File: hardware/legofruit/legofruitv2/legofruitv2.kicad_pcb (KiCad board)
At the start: 2 copper layers, 7.5 x 2 mm, 47 parts, among them J1 Conn_01x06, J10 SERVO4, J11 Conn_01x03, J12 MOTOR1, J2 USB_B_Micro, J3 Conn_ARM_JTAG_SWD_10, J4 MOTOR2, J5 SERVO1, J6 SERVO2, J7 SERVO3, J8 UART, J9 POWER, Q1 DMG2305, U1 MDBT50Q-1MV2, U2 MOTOR2_DRV, U4 AP2112K-3.3, U5 MOTOR1_DRV, Y1 32768 KHz

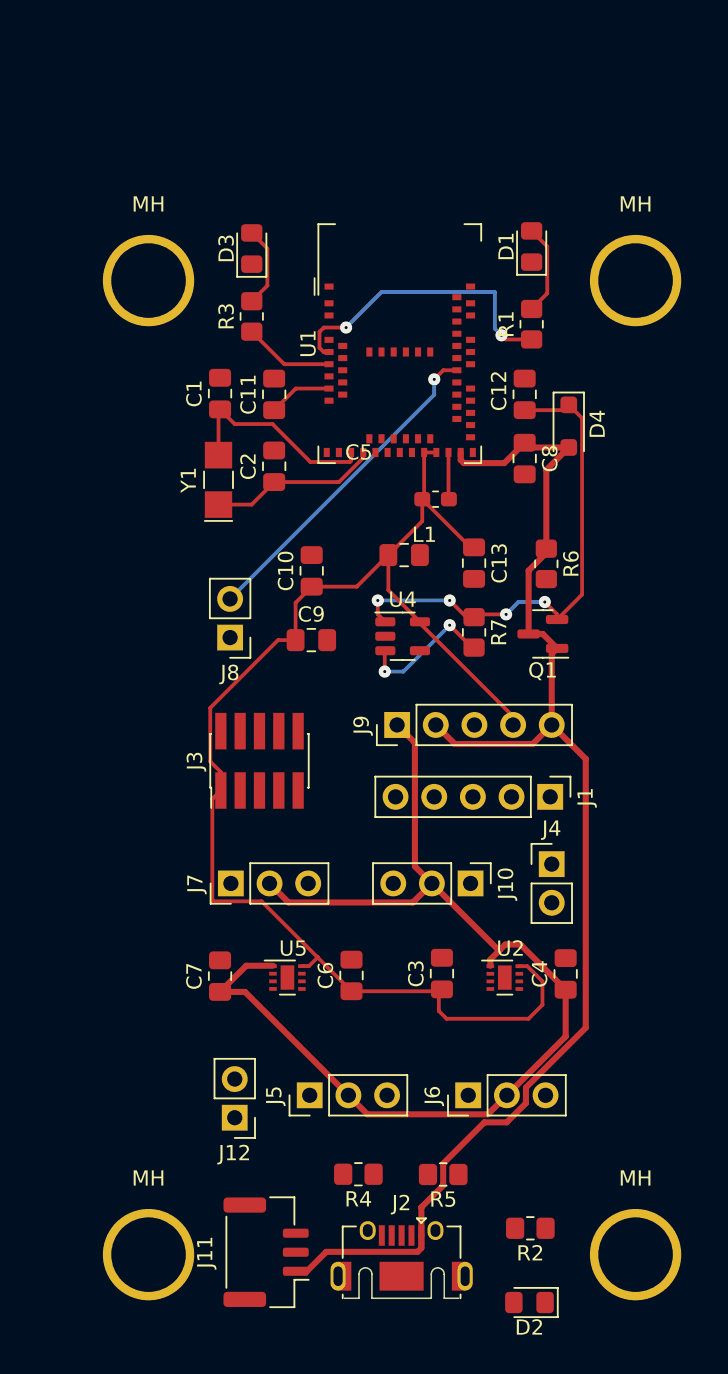
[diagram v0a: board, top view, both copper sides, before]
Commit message: Device driver version
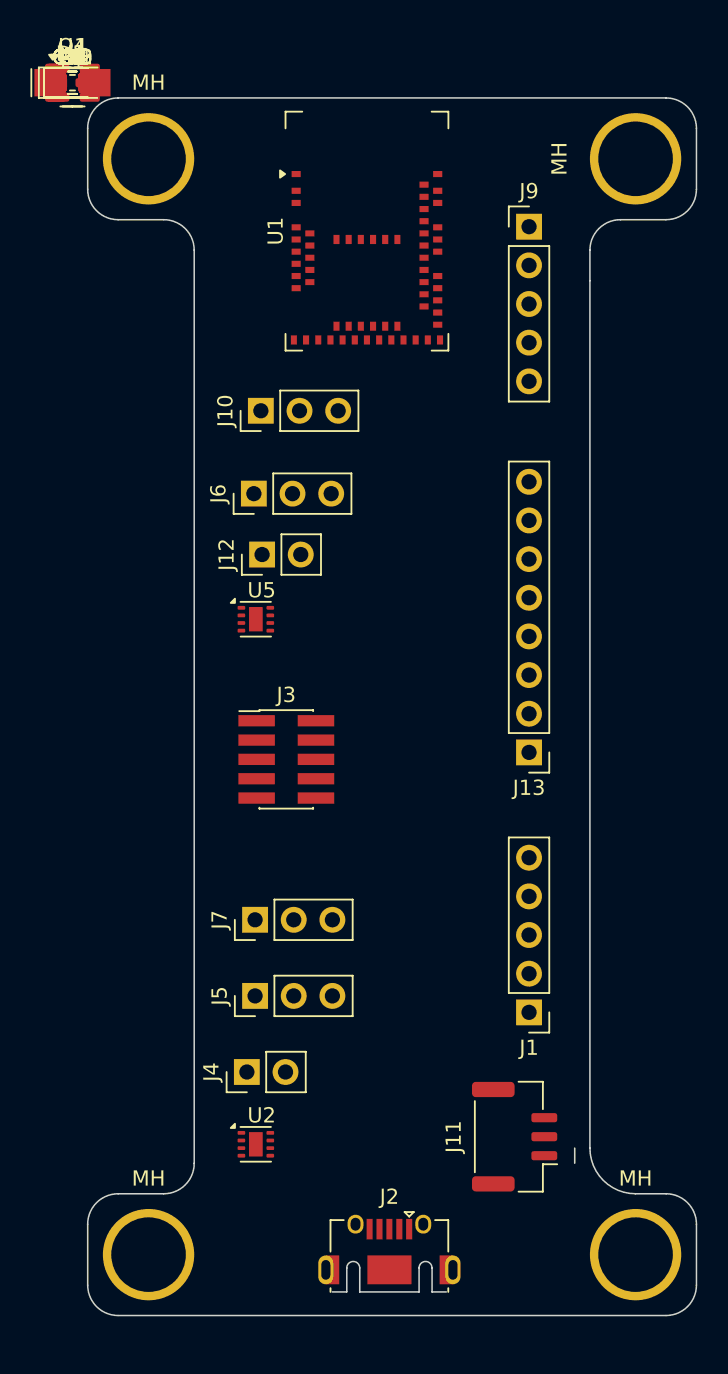
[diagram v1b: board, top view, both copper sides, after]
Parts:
- removed J8: UART, Connector_PinHeader_2.54mm:PinHeader_1x02_P2.54mm_Vertical
- added J13: GPIO, Connector_PinHeader_2.54mm:PinHeader_1x08_P2.54mm_Vertical, F.Cu at (125.0, 81.0)
- moved D2 85.6 mm to (95.0, 37.0), turned to 0 degrees
- moved R2 81.1 mm to (95.0, 37.0), turned to 0 degrees
- moved R5 75.8 mm to (95.0, 37.0), turned to 0 degrees
- moved R4 74.1 mm to (95.0, 37.0), turned to 0 degrees
- moved C4 66.9 mm to (95.0, 37.0), turned to 0 degrees
- moved C3 63.4 mm to (95.0, 37.0), turned to 0 degrees
- moved C6 61.5 mm to (95.0, 37.0), turned to 0 degrees
- moved C7 59.5 mm to (95.0, 37.0), turned to 0 degrees
- moved Q1 47.6 mm to (95.0, 37.0), turned to 0 degrees
- moved R7 44.7 mm to (95.0, 37.0), turned to 0 degrees
- moved R6 44.4 mm to (95.0, 37.0), turned to 0 degrees
- moved U4 42.3 mm to (95.0, 37.0)
- moved J6 42.0 mm to (106.9, 64.0)
- moved C13 41.1 mm to (95.0, 37.0), turned to 0 degrees
- moved C9 39.8 mm to (95.0, 37.0)
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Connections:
- U1 pad 43: Net-(J8-Pin_2) -> unconnected-(U1-P0.21-Pad43)
- U1 pad 44: Net-(J8-Pin_1) -> unconnected-(U1-P0.20-Pad44)
- U1 pad 50: unconnected-(U1-P1.02-Pad50) -> Net-(J13-Pin_5)
- U1 pad 56: unconnected-(U1-P1.04-Pad56) -> Net-(J13-Pin_3)
- U1 pad 57: unconnected-(U1-P1.06-Pad57) -> Net-(J13-Pin_1)
- U1 pad 59: unconnected-(U1-P1.05-Pad59) -> Net-(J13-Pin_2)
- U1 pad 60: unconnected-(U1-P1.03-Pad60) -> Net-(J13-Pin_4)
- U1 pad 61: unconnected-(U1-P1.01-Pad61) -> Net-(J13-Pin_6)
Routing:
- net +3.3V: track 89.5 -> 0.00 mm
- net VBUS: track 87.3 -> 0.00 mm
- net VCC: track 71.8 -> 0.00 mm
- net Net-(D4-K): track 33.1 -> 0.00 mm, vias 4 -> 0
- net Net-(J8-Pin_2): track 21.7 -> 0.00 mm, vias 1 -> 0
- net /P1.13: track 19.5 -> 0.00 mm, vias 2 -> 0
- net /XL1: track 13.7 -> 0.00 mm
- net /XL2: track 11.1 -> 0.00 mm
- net Net-(U4-EN): track 9.13 -> 0.00 mm, vias 2 -> 0
- net Net-(D1-A): track 5.98 -> 0.00 mm
- net /P1.15: track 5.96 -> 0.00 mm
- net Net-(D3-A): track 5.34 -> 0.00 mm
- net /AREF: track 4.19 -> 0.00 mm
- net Net-(U1-DCCH): track 3.08 -> 0.00 mm
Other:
- board size 7.5 x 2 mm -> 40 x 80 mm
